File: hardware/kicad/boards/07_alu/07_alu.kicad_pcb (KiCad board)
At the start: 2 copper layers, 104 parts, among them J1 Conn_01x08_Pin, J2 Conn_01x08_Pin, J3 Conn_01x08_Pin, J4 Conn_01x08_Pin, J5 Conn_01x08_Pin, J6 Conn_01x08_Pin, J7 Conn_01x16, SW1 SW_Slide_DPDT, U1 74ACT151, U10 74ACT151, U11 74ACT151, U12 74ACT151, U13 74ACT151, U14 74ACT151, U15 74ACT283, U16 74LS32, U17 74ACT151, U18 74ACT151, U19 74ACT151, U2 74ACT151, U20 74ACT151, U21 74ACT151, U22 74ACT151, U23 74ACT151, U24 74ACT151, U25 74ACT283, U26 74LS32, U27 74ACT151, U28 74ACT151, U29 74ACT151, U3 74ACT283, U30 74ACT151, U31 74ACT151, U32 74ACT151, U33 74ACT151, U34 74ACT151, U35 SST39SF040, U36 SST39SF040, U37 74AHC541, U38 74AHC541, U39 SST39SF040, U4 74LS32, U40 74AHC541, U41 74ACT151, U42 74ACT151, U43 74ACT151, U44 74ACT151, U45 74ACT151, U46 74ACT151, U47 74ACT151, U48 74ACT151, U5 74ACT283, U6 74LS32, U7 74ACT151, U8 74ACT151, U9 74ACT151

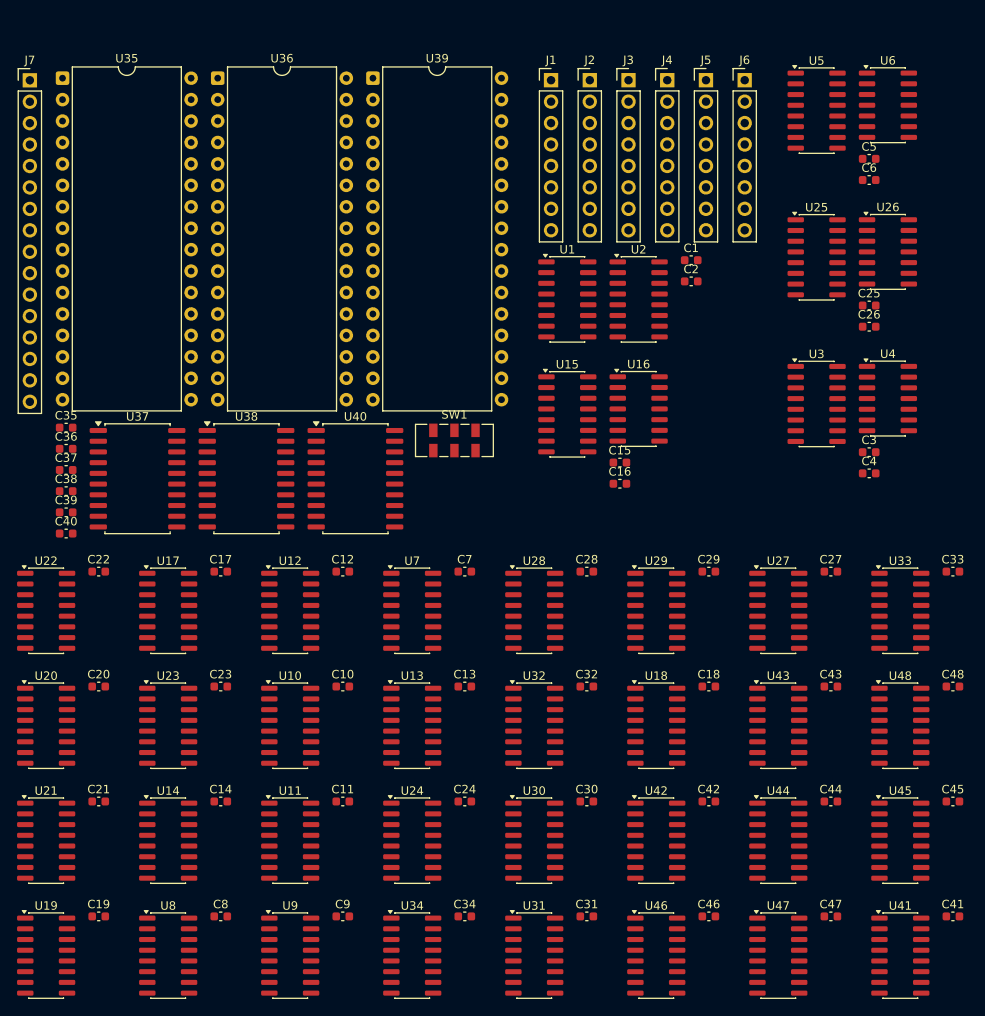
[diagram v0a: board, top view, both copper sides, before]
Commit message: checkpoint: most recent 16b cell: ~120mm by 120mm
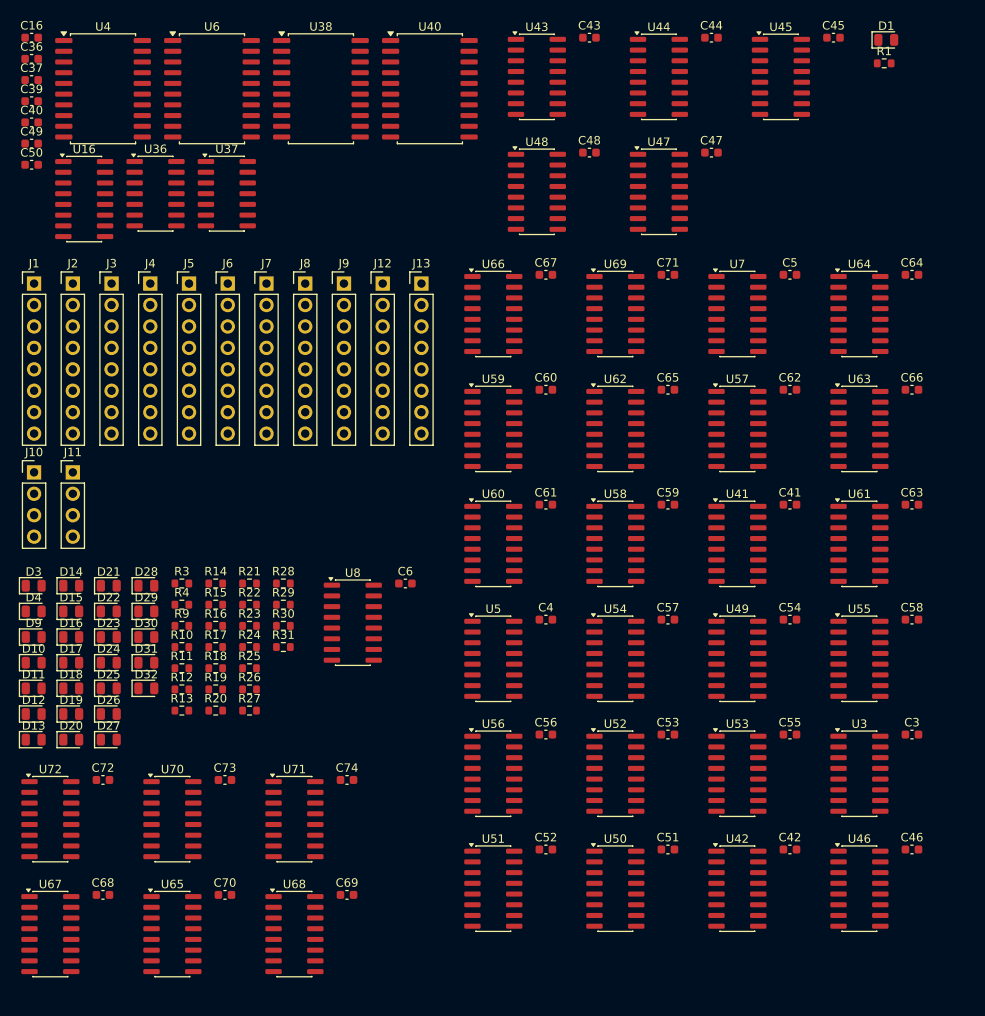
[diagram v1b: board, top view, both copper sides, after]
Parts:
- removed C1, C10, C11, C12, C13, C14, C15, C17, C18, C19, C2, C20, C21, C22, C23, C24, C25, C26, C27, C28, C29, C30, C31, C32, C33, C34, C35, C38, C7, C8, C9: 100nF, Capacitor_SMD:C_0603_1608Metric
- removed SW1: SW_Slide_DPDT, Button_Switch_SMD:SW_DPDT_CK_JS202011JCQN
- removed U1, U10, U11, U12, U13, U14, U17, U18, U19, U2, U20, U21, U22, U23, U24, U27, U28, U29, U30, U31, U32, U33, U34, U9: 74ACT151, Package_SO:SOIC-16_3.9x9.9mm_P1.27mm
- removed U15, U25: 74ACT283, Package_SO:SOIC-16_3.9x9.9mm_P1.27mm
- removed U26: 74LS32, Package_SO:SOIC-14_3.9x8.7mm_P1.27mm
- removed U35, U39: SST39SF040, Package_DIP:DIP-32_W15.24mm
- added C49: 100nF, Capacitor_SMD:C_0603_1608Metric, F.Cu at (57.5, 41.8)
- added C50: 100nF, Capacitor_SMD:C_0603_1608Metric, F.Cu at (57.5, 44.3)
- added C51: 100nF, Capacitor_SMD:C_0603_1608Metric, F.Cu at (132.9, 125.5)
- added C52: 100nF, Capacitor_SMD:C_0603_1608Metric, F.Cu at (118.4, 125.5)
- added C53: 100nF, Capacitor_SMD:C_0603_1608Metric, F.Cu at (132.9, 111.8)
- added C54: 100nF, Capacitor_SMD:C_0603_1608Metric, F.Cu at (147.4, 98.2)
- added C55: 100nF, Capacitor_SMD:C_0603_1608Metric, F.Cu at (147.4, 111.8)
- added C56: 100nF, Capacitor_SMD:C_0603_1608Metric, F.Cu at (118.4, 111.8)
- added C57: 100nF, Capacitor_SMD:C_0603_1608Metric, F.Cu at (132.9, 98.2)
- added C58: 100nF, Capacitor_SMD:C_0603_1608Metric, F.Cu at (161.8, 98.2)
- added C59: 100nF, Capacitor_SMD:C_0603_1608Metric, F.Cu at (132.9, 84.6)
- added C60: 100nF, Capacitor_SMD:C_0603_1608Metric, F.Cu at (118.4, 71.0)
- added C61: 100nF, Capacitor_SMD:C_0603_1608Metric, F.Cu at (118.4, 84.6)
- added C62: 100nF, Capacitor_SMD:C_0603_1608Metric, F.Cu at (147.4, 71.0)
- added C63: 100nF, Capacitor_SMD:C_0603_1608Metric, F.Cu at (161.8, 84.6)
- added C64: 100nF, Capacitor_SMD:C_0603_1608Metric, F.Cu at (161.8, 57.4)
- added C65: 100nF, Capacitor_SMD:C_0603_1608Metric, F.Cu at (132.9, 71.0)
- added C66: 100nF, Capacitor_SMD:C_0603_1608Metric, F.Cu at (161.8, 71.0)
- added C67: 100nF, Capacitor_SMD:C_0603_1608Metric, F.Cu at (118.4, 57.4)
- added C68: 100nF, Capacitor_SMD:C_0603_1608Metric, F.Cu at (66.0, 130.8)
- added C69: 100nF, Capacitor_SMD:C_0603_1608Metric, F.Cu at (94.9, 130.8)
- added C70: 100nF, Capacitor_SMD:C_0603_1608Metric, F.Cu at (80.4, 130.8)
- added C71: 100nF, Capacitor_SMD:C_0603_1608Metric, F.Cu at (132.9, 57.4)
- added C72: 100nF, Capacitor_SMD:C_0603_1608Metric, F.Cu at (66.0, 117.2)
- added C73: 100nF, Capacitor_SMD:C_0603_1608Metric, F.Cu at (80.4, 117.2)
- added C74: 100nF, Capacitor_SMD:C_0603_1608Metric, F.Cu at (94.9, 117.2)
- added D1: LED, LED_SMD:LED_0805_2012Metric, F.Cu at (158.8, 29.5)
- added D10: LED, LED_SMD:LED_0805_2012Metric, F.Cu at (57.7, 103.3)
- added D11: LED, LED_SMD:LED_0805_2012Metric, F.Cu at (57.7, 106.4)
- added D12: LED, LED_SMD:LED_0805_2012Metric, F.Cu at (57.7, 109.4)
- added D13: LED, LED_SMD:LED_0805_2012Metric, F.Cu at (57.7, 112.4)
- added D14: LED, LED_SMD:LED_0805_2012Metric, F.Cu at (62.2, 94.2)
- added D15: LED, LED_SMD:LED_0805_2012Metric, F.Cu at (62.2, 97.2)
- added D16: LED, LED_SMD:LED_0805_2012Metric, F.Cu at (62.2, 100.3)
- added D17: LED, LED_SMD:LED_0805_2012Metric, F.Cu at (62.2, 103.3)
- added D18: LED, LED_SMD:LED_0805_2012Metric, F.Cu at (62.2, 106.4)
- added D19: LED, LED_SMD:LED_0805_2012Metric, F.Cu at (62.2, 109.4)
- added D20: LED, LED_SMD:LED_0805_2012Metric, F.Cu at (62.2, 112.4)
- added D21: LED, LED_SMD:LED_0805_2012Metric, F.Cu at (66.6, 94.2)
- added D22: LED, LED_SMD:LED_0805_2012Metric, F.Cu at (66.6, 97.2)
- added D23: LED, LED_SMD:LED_0805_2012Metric, F.Cu at (66.6, 100.3)
- added D24: LED, LED_SMD:LED_0805_2012Metric, F.Cu at (66.6, 103.3)
- added D25: LED, LED_SMD:LED_0805_2012Metric, F.Cu at (66.6, 106.4)
- added D26: LED, LED_SMD:LED_0805_2012Metric, F.Cu at (66.6, 109.4)
- added D27: LED, LED_SMD:LED_0805_2012Metric, F.Cu at (66.6, 112.4)
- added D28: LED, LED_SMD:LED_0805_2012Metric, F.Cu at (71.1, 94.2)
- added D29: LED, LED_SMD:LED_0805_2012Metric, F.Cu at (71.1, 97.2)
- added D3: LED, LED_SMD:LED_0805_2012Metric, F.Cu at (57.7, 94.2)
- added D30: LED, LED_SMD:LED_0805_2012Metric, F.Cu at (71.1, 100.3)
- added D31: LED, LED_SMD:LED_0805_2012Metric, F.Cu at (71.1, 103.3)
- added D32: LED, LED_SMD:LED_0805_2012Metric, F.Cu at (71.1, 106.4)
- added D4: LED, LED_SMD:LED_0805_2012Metric, F.Cu at (57.7, 97.2)
- added D9: LED, LED_SMD:LED_0805_2012Metric, F.Cu at (57.7, 100.3)
- added J10: Conn_01x04_Pin, Connector_PinHeader_2.54mm:PinHeader_1x04_P2.54mm_Vertical, F.Cu at (57.8, 80.8)
- added J11: Conn_01x04_Pin, Connector_PinHeader_2.54mm:PinHeader_1x04_P2.54mm_Vertical, F.Cu at (62.4, 80.8)
- added J12: Conn_01x08_Pin, Connector_PinHeader_2.54mm:PinHeader_1x08_P2.54mm_Vertical, F.Cu at (99.1, 58.4)
- added J13: Conn_01x08_Pin, Connector_PinHeader_2.54mm:PinHeader_1x08_P2.54mm_Vertical, F.Cu at (103.7, 58.4)
- added J8: Conn_01x08_Pin, Connector_PinHeader_2.54mm:PinHeader_1x08_P2.54mm_Vertical, F.Cu at (89.9, 58.4)
- added J9: Conn_01x08_Pin, Connector_PinHeader_2.54mm:PinHeader_1x08_P2.54mm_Vertical, F.Cu at (94.5, 58.4)
- added R1: 330 Ohm, Resistor_SMD:R_0603_1608Metric, F.Cu at (158.5, 32.3)
- added R10: 330, Resistor_SMD:R_0603_1608Metric, F.Cu at (75.3, 101.5)
- added R11: 330, Resistor_SMD:R_0603_1608Metric, F.Cu at (75.3, 104.0)
- added R12: 330, Resistor_SMD:R_0603_1608Metric, F.Cu at (75.3, 106.5)
- added R13: 330, Resistor_SMD:R_0603_1608Metric, F.Cu at (75.3, 109.0)
- added R14: 330, Resistor_SMD:R_0603_1608Metric, F.Cu at (79.3, 93.9)
- added R15: 330, Resistor_SMD:R_0603_1608Metric, F.Cu at (79.3, 96.4)
- added R16: 330, Resistor_SMD:R_0603_1608Metric, F.Cu at (79.3, 99.0)
- added R17: 330, Resistor_SMD:R_0603_1608Metric, F.Cu at (79.3, 101.5)
- added R18: 330, Resistor_SMD:R_0603_1608Metric, F.Cu at (79.3, 104.0)
- added R19: 330, Resistor_SMD:R_0603_1608Metric, F.Cu at (79.3, 106.5)
- added R20: 330, Resistor_SMD:R_0603_1608Metric, F.Cu at (79.3, 109.0)
- added R21: 330, Resistor_SMD:R_0603_1608Metric, F.Cu at (83.3, 93.9)
- added R22: 330, Resistor_SMD:R_0603_1608Metric, F.Cu at (83.3, 96.4)
- added R23: 330, Resistor_SMD:R_0603_1608Metric, F.Cu at (83.3, 99.0)
- added R24: 330, Resistor_SMD:R_0603_1608Metric, F.Cu at (83.3, 101.5)
- added R25: 330, Resistor_SMD:R_0603_1608Metric, F.Cu at (83.3, 104.0)
- added R26: 330, Resistor_SMD:R_0603_1608Metric, F.Cu at (83.3, 106.5)
- added R27: 330, Resistor_SMD:R_0603_1608Metric, F.Cu at (83.3, 109.0)
- added R28: 330, Resistor_SMD:R_0603_1608Metric, F.Cu at (87.3, 93.9)
- added R29: 330, Resistor_SMD:R_0603_1608Metric, F.Cu at (87.3, 96.4)
- added R3: 330 Ohm, Resistor_SMD:R_0603_1608Metric, F.Cu at (75.3, 93.9)
- added R30: 330, Resistor_SMD:R_0603_1608Metric, F.Cu at (87.3, 99.0)
- added R31: 330, Resistor_SMD:R_0603_1608Metric, F.Cu at (87.3, 101.5)
- added R4: 330, Resistor_SMD:R_0603_1608Metric, F.Cu at (75.3, 96.4)
- added R9: 330, Resistor_SMD:R_0603_1608Metric, F.Cu at (75.3, 99.0)
- added U49: 74ACT151, Package_SO:SOIC-16_3.9x9.9mm_P1.27mm, F.Cu at (141.1, 102.9)
- added U50: 74ACT151, Package_SO:SOIC-16_3.9x9.9mm_P1.27mm, F.Cu at (126.7, 130.1)
- added U51: 74ACT151, Package_SO:SOIC-16_3.9x9.9mm_P1.27mm, F.Cu at (112.2, 130.1)
- added U52: 74ACT151, Package_SO:SOIC-16_3.9x9.9mm_P1.27mm, F.Cu at (126.7, 116.5)
- added U53: 74ACT151, Package_SO:SOIC-16_3.9x9.9mm_P1.27mm, F.Cu at (141.1, 116.5)
- added U54: 74ACT151, Package_SO:SOIC-16_3.9x9.9mm_P1.27mm, F.Cu at (126.7, 102.9)
- added U55: 74ACT151, Package_SO:SOIC-16_3.9x9.9mm_P1.27mm, F.Cu at (155.6, 102.9)
- added U56: 74ACT151, Package_SO:SOIC-16_3.9x9.9mm_P1.27mm, F.Cu at (112.2, 116.5)
- added U57: 74ACT151, Package_SO:SOIC-16_3.9x9.9mm_P1.27mm, F.Cu at (141.1, 75.6)
- added U58: 74ACT151, Package_SO:SOIC-16_3.9x9.9mm_P1.27mm, F.Cu at (126.7, 89.2)
- added U59: 74ACT151, Package_SO:SOIC-16_3.9x9.9mm_P1.27mm, F.Cu at (112.2, 75.6)
- added U60: 74ACT151, Package_SO:SOIC-16_3.9x9.9mm_P1.27mm, F.Cu at (112.2, 89.2)
- added U61: 74ACT151, Package_SO:SOIC-16_3.9x9.9mm_P1.27mm, F.Cu at (155.6, 89.2)
- added U62: 74ACT151, Package_SO:SOIC-16_3.9x9.9mm_P1.27mm, F.Cu at (126.7, 75.6)
- added U63: 74ACT151, Package_SO:SOIC-16_3.9x9.9mm_P1.27mm, F.Cu at (155.6, 75.6)
- added U64: 74ACT151, Package_SO:SOIC-16_3.9x9.9mm_P1.27mm, F.Cu at (155.6, 62.0)
- added U65: 74ACT151, Package_SO:SOIC-16_3.9x9.9mm_P1.27mm, F.Cu at (74.2, 135.5)
- added U66: 74ACT151, Package_SO:SOIC-16_3.9x9.9mm_P1.27mm, F.Cu at (112.2, 62.0)
- added U67: 74ACT151, Package_SO:SOIC-16_3.9x9.9mm_P1.27mm, F.Cu at (59.7, 135.5)
- added U68: 74ACT151, Package_SO:SOIC-16_3.9x9.9mm_P1.27mm, F.Cu at (88.6, 135.5)
- added U69: 74ACT151, Package_SO:SOIC-16_3.9x9.9mm_P1.27mm, F.Cu at (126.7, 62.0)
- added U70: 74ACT151, Package_SO:SOIC-16_3.9x9.9mm_P1.27mm, F.Cu at (74.2, 121.9)
- added U71: 74ACT151, Package_SO:SOIC-16_3.9x9.9mm_P1.27mm, F.Cu at (88.6, 121.9)
- added U72: 74ACT151, Package_SO:SOIC-16_3.9x9.9mm_P1.27mm, F.Cu at (59.7, 121.9)
- J7: value Conn_01x16 -> Conn_01x08_Pin; footprint Connector_PinHeader_2.54mm:PinHeader_1x16_P2.54mm_Vertical -> Connector_PinHeader_2.54mm:PinHeader_1x08_P2.54mm_Vertical
- U16: value 74LS32 -> 74ACT151; footprint Package_SO:SOIC-14_3.9x8.7mm_P1.27mm -> Package_SO:SOIC-16_3.9x9.9mm_P1.27mm
- U36: value SST39SF040 -> 74HC86; footprint Package_DIP:DIP-32_W15.24mm -> Package_SO:SOIC-14_3.9x8.7mm_P1.27mm
- U37: value 74AHC541 -> 74LS08; footprint Package_SO:SOIC-20W_7.5x12.8mm_P1.27mm -> Package_SO:SOIC-14_3.9x8.7mm_P1.27mm
- U38: value 74AHC541 -> 74LS540
- U4, U6: value 74LS32 -> 74HC688; footprint Package_SO:SOIC-14_3.9x8.7mm_P1.27mm -> Package_SO:SOIC-20W_7.5x12.8mm_P1.27mm
- U40: value 74AHC541 -> 74LS377
- U7, U8: value 74ACT151 -> 74ACT283
- moved U4 100.0 mm to (66.0, 35.3)
- moved C44 91.6 mm to (138.1, 29.3)
- moved C45 91.6 mm to (152.5, 29.3)
- moved C47 91.6 mm to (138.1, 42.9)
- moved U44 91.6 mm to (131.8, 33.9)
- moved U45 91.6 mm to (146.3, 33.9)
- moved U47 91.6 mm to (131.8, 47.5)
- moved C16 87.5 mm to (57.5, 29.3)
- moved U43 82.0 mm to (117.4, 33.9)
- moved C43 82.0 mm to (123.6, 29.3)
- moved U6 80.1 mm to (78.9, 35.3)
- moved C48 76.5 mm to (123.6, 42.9)
- moved U48 76.5 mm to (117.4, 47.5)
- moved U5 75.4 mm to (112.2, 102.9)
- moved C6 72.8 mm to (101.8, 93.9)
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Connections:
- C36 pad 1: VCC -> GND
- C36 pad 2: GND -> VCC
- C37 pad 1: VCC -> GND
- C37 pad 2: GND -> VCC
- C39 pad 1: VCC -> GND
- C39 pad 2: GND -> VCC
- J7 pad 1: OPCODE0 -> ALU_OPCODE_Y0
- J7 pad 2: OPCODE1 -> ALU_OPCODE_Y1
- J7 pad 3: OPCODE2 -> ALU_OPCODE_Y2
- J7 pad 4: OPCODE3 -> ALU_OPCODE_Y3
- J7 pad 5: OPCODE4 -> ALU_OPCODE_Y4
- J7 pad 6: OPCODE5 -> ALU_OPCODE_Y5
- J7 pad 7: OPCODE6 -> ALU_OPCODE_Y6
- J7 pad 8: OPCODE7 -> ALU_OPCODE_Y7
- U16 pad 1: OUT8 -> flagZ
- U16 pad 10: Net-(U16-Pad10) -> CSEL1
- U16 pad 11: /alu_4b_2/Z_out -> CSEL0
- U16 pad 12: Net-(U16-Pad12) -> flagGT
- U16 pad 13: /alu_4b_1/Z_out -> flagLT
- U16 pad 14: VCC -> flagV
- U16 pad 2: OUT9 -> flagC
- U16 pad 3: Net-(U16-Pad3) -> VCC
- U16 pad 4: OUT10 -> GND
- U16 pad 5: OUT11 -> CIN-MAIN
- U16 pad 6: Net-(U16-Pad10) -> unconnected-(U16-~{Z}-Pad6)
- U16 pad 8: Net-(U16-Pad12) -> GND
- U16 pad 9: Net-(U16-Pad3) -> CSEL2
- U3 pad 7: CIN -> CIN-MAIN
- U36 pad 1: GND -> Aeff
- U36 pad 10: OPCODE2 -> VOUT
- U36 pad 11: OPCODE1 -> unconnected-(U36-Pad11)
- U36 pad 12: OPCODE0 -> unconnected-(U36-Pad12)
- U36 pad 13: Net-(U36-D0) -> unconnected-(U36-Pad13)
- U36 pad 14: Net-(U36-D1) -> VCC
- U36 pad 2: GND -> sum15
- U36 pad 3: OPCODE15 -> Net-(U36-Pad3)
- U36 pad 4: OPCODE12 -> sum15
- U36 pad 5: OPCODE7 -> Beff
- U36 pad 6: OPCODE6 -> Net-(U36-Pad6)
- U36 pad 7: OPCODE5 -> GND
- U36 pad 8: OPCODE4 -> LT-SIGN
- U36 pad 9: OPCODE3 -> OUT15
- U37 pad 1: GND -> Net-(U36-Pad3)
- U37 pad 10: GND -> unconnected-(U37-Pad10)
- U37 pad 11: CTRL2 -> GT-SIGN
- U37 pad 12: CTRL1 -> GTE-SIGN
- U37 pad 13: CTRL0 -> ~ZOUT
- U37 pad 14: FLAG_WE -> VCC
- U37 pad 2: Net-(U36-D0) -> Net-(U36-Pad6)
- U37 pad 3: Net-(U36-D1) -> VOUT
- U37 pad 4: Net-(U36-D2) -> unconnected-(U37-Pad4)
- U37 pad 5: Net-(U36-D3) -> unconnected-(U37-Pad5)
- U37 pad 6: Net-(U36-D4) -> unconnected-(U37-Pad6)
- U37 pad 7: Net-(U36-D5) -> GND
- U37 pad 8: Net-(U36-D6) -> unconnected-(U37-Pad8)
- U37 pad 9: Net-(U36-D7) -> unconnected-(U37-Pad9)
- U38 pad 11: ALU_OPCODE_X7 -> unconnected-(U38-Y7-Pad11)
- U38 pad 12: ALU_OPCODE_X6 -> unconnected-(U38-Y6-Pad12)
- U38 pad 13: ALU_OPCODE_X5 -> ~flagWE
- U38 pad 14: ALU_OPCODE_X4 -> unconnected-(U38-Y4-Pad14)
- U38 pad 15: ALU_OPCODE_X3 -> GTE-SIGN
- U38 pad 16: ALU_OPCODE_X2 -> unconnected-(U38-Y2-Pad16)
- U38 pad 17: ALU_OPCODE_X1 -> unconnected-(U38-Y1-Pad17)
- U38 pad 18: ALU_OPCODE_X0 -> ZOUT
- U38 pad 2: Net-(U35-D0) -> ~ZOUT
- U38 pad 3: Net-(U35-D1) -> unconnected-(U38-A1-Pad3)
- U38 pad 4: Net-(U35-D2) -> VOUT
- U38 pad 5: Net-(U35-D3) -> LT-SIGN
- U38 pad 6: Net-(U35-D4) -> OUT15
- U38 pad 7: Net-(U35-D5) -> FLAG_WE
- U38 pad 8: Net-(U35-D6) -> unconnected-(U38-A6-Pad8)
- U38 pad 9: Net-(U35-D7) -> unconnected-(U38-A7-Pad9)
- U4 pad 1: OUT0 -> GND
- U4 pad 10: Net-(U4-Pad10) -> GND
- U4 pad 11: /alu_4b_0/Z_out -> OUT4
- U4 pad 12: Net-(U4-Pad12) -> GND
- U4 pad 13: /alu_4b_0/Z_in -> OUT5
- U4 pad 14: VCC -> GND
- U4 pad 2: OUT1 -> OUT0
- U4 pad 3: Net-(U4-Pad3) -> GND
- U4 pad 4: OUT2 -> OUT1
- U4 pad 5: OUT3 -> GND
- U4 pad 6: Net-(U4-Pad10) -> OUT2
- U4 pad 8: Net-(U4-Pad12) -> OUT3
- U4 pad 9: Net-(U4-Pad3) -> GND
- U40 pad 1: GND -> ~flagWE
- U40 pad 11: ALU_OPCODE_Y7 -> SYS-CLK
- U40 pad 12: ALU_OPCODE_Y6 -> flagV
- U40 pad 13: ALU_OPCODE_Y5 -> VOUT
- U40 pad 14: ALU_OPCODE_Y4 -> LT-SIGN
- U40 pad 15: ALU_OPCODE_Y3 -> flagLT
- U40 pad 16: ALU_OPCODE_Y2 -> flagGT
- U40 pad 17: ALU_OPCODE_Y1 -> GT-SIGN
- U40 pad 18: ALU_OPCODE_Y0 -> GTE-SIGN
- U40 pad 19: GND -> flagGTE
- U40 pad 2: Net-(U39-D0) -> flagZ
- U40 pad 3: Net-(U39-D1) -> ZOUT
- U40 pad 4: Net-(U39-D2) -> ~ZOUT
- U40 pad 5: Net-(U39-D3) -> ~flagZ
- U40 pad 6: Net-(U39-D4) -> flagN
- U40 pad 7: Net-(U39-D5) -> OUT15
- U40 pad 8: Net-(U39-D6) -> COUT-MAIN
- U40 pad 9: Net-(U39-D7) -> flagC
- U6 pad 1: OUT4 -> Net-(U4-P=R)
- U6 pad 10: Net-(U6-Pad10) -> GND
- U6 pad 11: /alu_4b_1/Z_out -> OUT12
- U6 pad 12: Net-(U6-Pad12) -> GND
- U6 pad 13: /alu_4b_0/Z_out -> OUT13
- U6 pad 14: VCC -> GND
- U6 pad 2: OUT5 -> OUT8
- U6 pad 3: Net-(U6-Pad3) -> GND
- U6 pad 4: OUT6 -> OUT9
- U6 pad 5: OUT7 -> GND
- U6 pad 6: Net-(U6-Pad10) -> OUT10
- U6 pad 8: Net-(U6-Pad12) -> OUT11
- U6 pad 9: Net-(U6-Pad3) -> GND
- U7 pad 1: ALU_OPCODE_X3 -> OUT9
- U7 pad 10: B4 -> OUT11
- U7 pad 11: A4 -> /alu_4b_2/logB3
- U7 pad 12: ALU_OPCODE_X7 -> /alu_4b_2/logA3
- U7 pad 13: ALU_OPCODE_X6 -> OUT10
- U7 pad 14: ALU_OPCODE_X5 -> /alu_4b_2/logA2
- U7 pad 15: ALU_OPCODE_X4 -> /alu_4b_2/logB2
- U7 pad 2: ALU_OPCODE_X2 -> /alu_4b_2/logB1
- U7 pad 3: ALU_OPCODE_X1 -> /alu_4b_2/logA1
- U7 pad 4: ALU_OPCODE_X0 -> OUT8
- U7 pad 5: /alu_4b_1/logA0 -> /alu_4b_2/logA0
- U7 pad 6: unconnected-(U7-~{Z}-Pad6) -> /alu_4b_2/logB0
- U7 pad 7: GND -> /alu_4b_1/cout
- U7 pad 9: C4 -> /alu_4b_2/cout
- U8 pad 1: ALU_OPCODE_X3 -> OUT13
- U8 pad 10: B5 -> sum15
- U8 pad 11: A5 -> Beff
- U8 pad 12: ALU_OPCODE_X7 -> Aeff
- U8 pad 13: ALU_OPCODE_X6 -> OUT14
- U8 pad 14: ALU_OPCODE_X5 -> /alu_4b_3/logA2
- U8 pad 15: ALU_OPCODE_X4 -> /alu_4b_3/logB2
- U8 pad 2: ALU_OPCODE_X2 -> /alu_4b_3/logB1
- U8 pad 3: ALU_OPCODE_X1 -> /alu_4b_3/logA1
- U8 pad 4: ALU_OPCODE_X0 -> OUT12
- U8 pad 5: /alu_4b_1/logA1 -> /alu_4b_3/logA0
- U8 pad 6: unconnected-(U8-~{Z}-Pad6) -> /alu_4b_3/logB0
- U8 pad 7: GND -> /alu_4b_2/cout
- U8 pad 9: C5 -> COUT-MAIN
